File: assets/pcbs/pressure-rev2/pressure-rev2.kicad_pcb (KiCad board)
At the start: 2 copper layers, 65 x 56 mm, 21 parts, among them J1 40HAT, J2 Conn_01x04, J3 Conn_02x01, J4 Conn_01x03, U1 TL7660, U2 INA126, U3 MINI-P-Sensor, U4 Adafruit_ADS1115, U5 MINI-P-Sensor, U6 MINI-P-Sensor

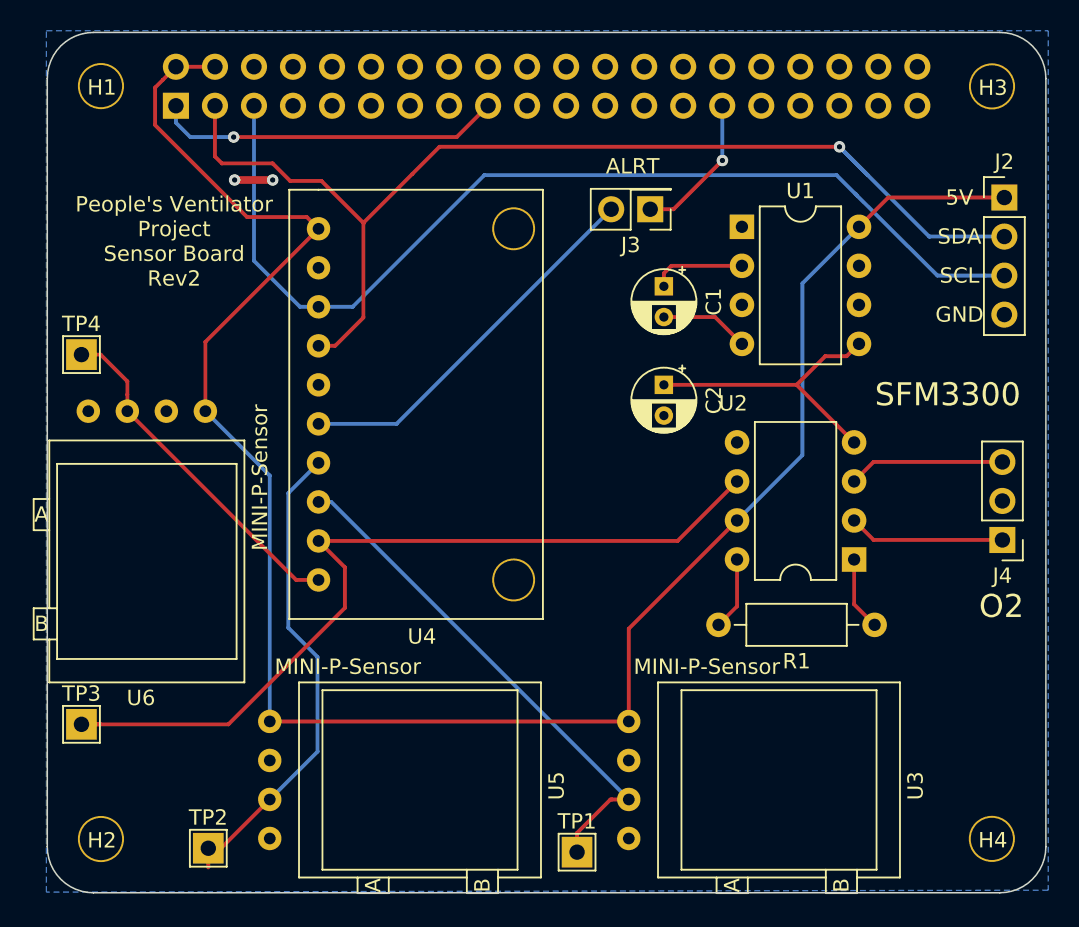
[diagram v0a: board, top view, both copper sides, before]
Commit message: revised, added schematic images
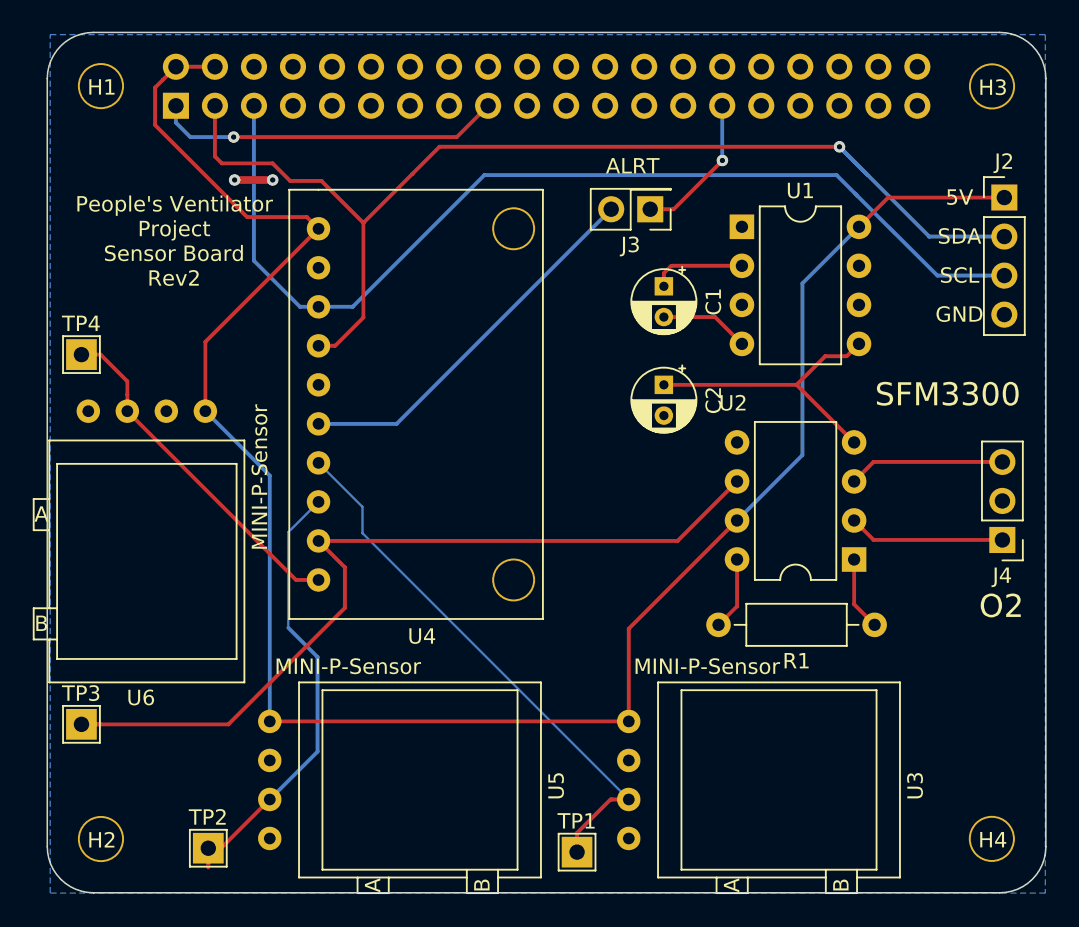
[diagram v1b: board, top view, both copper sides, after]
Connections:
- U4 pad 7: Net-(TP2-Pad1) -> Net-(TP1-Pad1)
- U4 pad 8: Net-(TP1-Pad1) -> Net-(TP2-Pad1)
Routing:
- net Net-(TP2-Pad1): track 31.4 -> 28.8 mm
- net Net-(TP1-Pad1): track 33.7 -> 35.8 mm
